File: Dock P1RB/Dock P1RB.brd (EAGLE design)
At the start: 41 x 46 mm, 16 parts, among them U1 MCP73831T-2ACI/OT

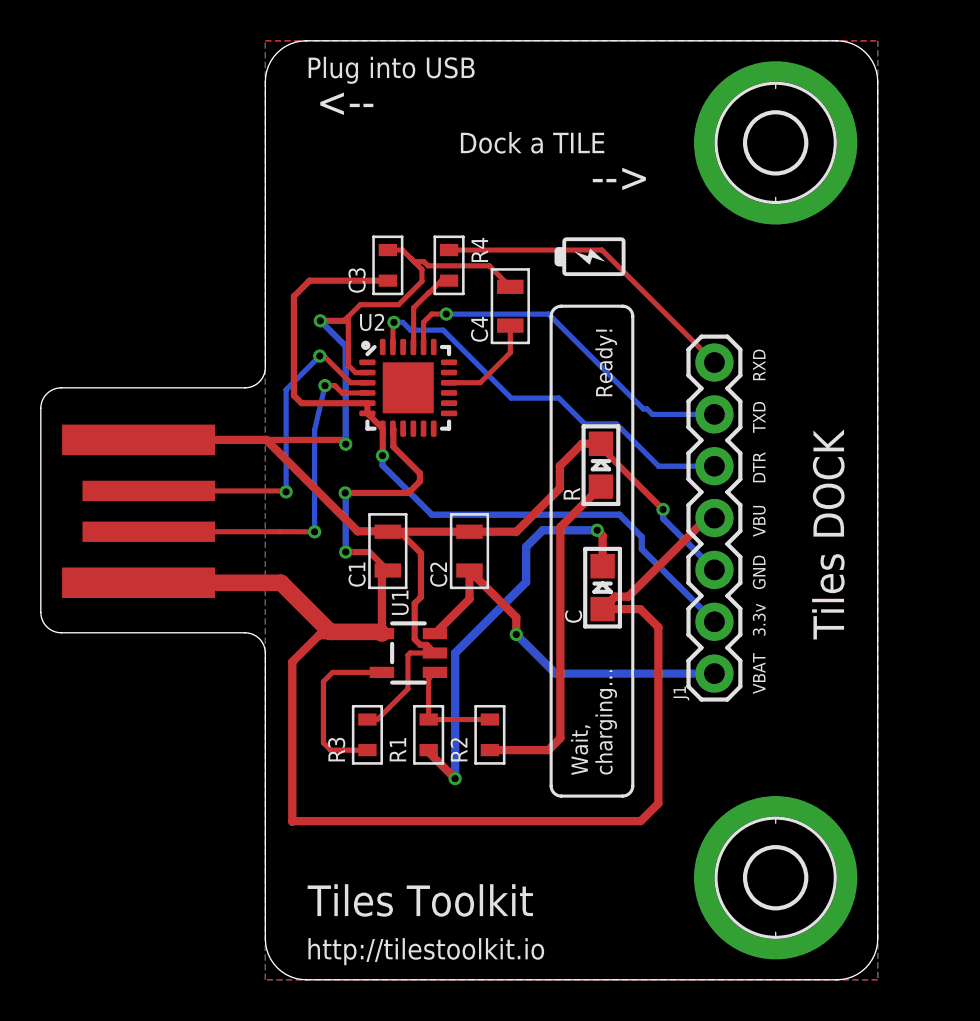
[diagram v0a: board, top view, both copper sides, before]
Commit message: dock ready for prod
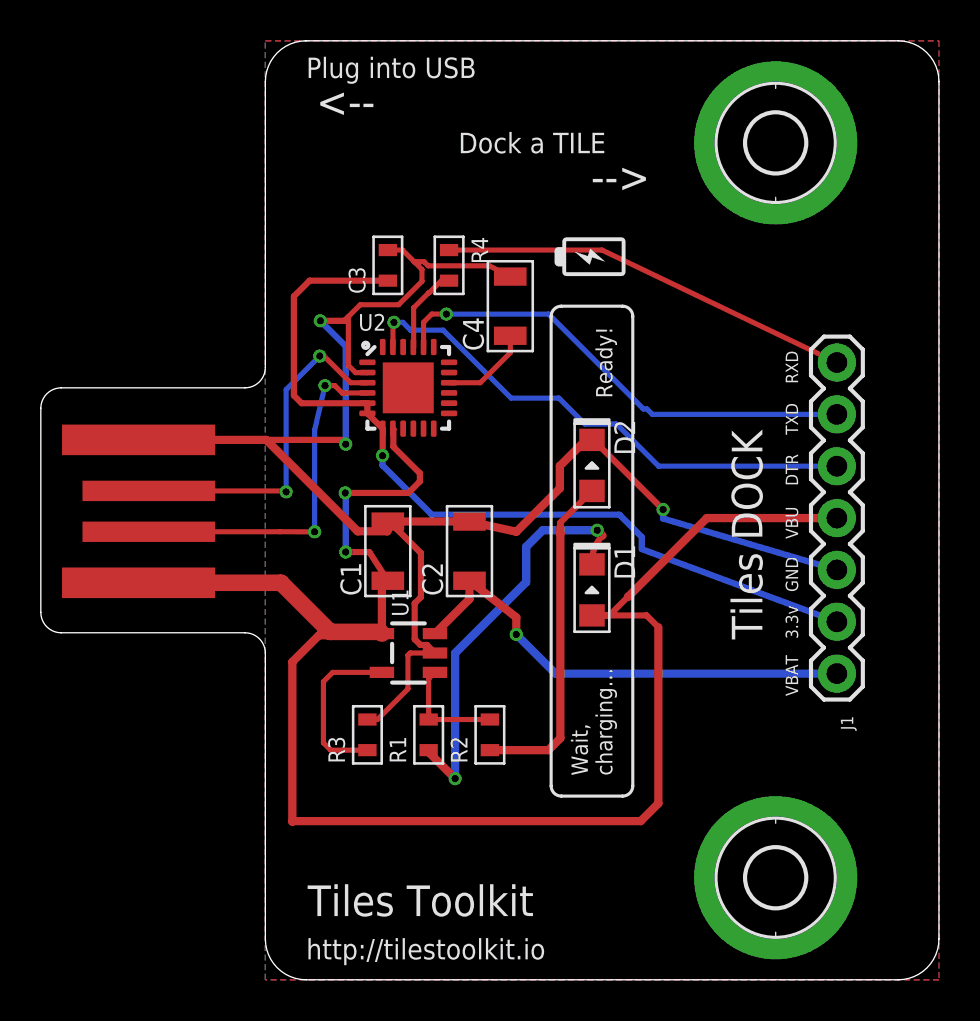
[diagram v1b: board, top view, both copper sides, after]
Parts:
- removed C: RED, microbuilder:CHIPLED_0805
- removed R: GREEN, microbuilder:CHIPLED_0805
- added D1: MF-LED-0805-RED, MF_LEDs:LED0805
- added D2: MF-LED-0805-GREEN, MF_LEDs:LED0805
- C1, C2, C4: device MF_Passives:C0805 -> MF_Passives:C1206
- moved J1 6.00 mm to (28.0, -31.0)
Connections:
- net GND: now also D2.CATHODE; no longer R.C
- net N$1: now also D1.CATHODE; no longer C.C
- net N$6: now also D2.ANODE; no longer R.A
- net VBUS: now also D1.ANODE; no longer C.A
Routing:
- net VBUS: track 76.2 -> 83.6 mm
- net TXD: track 17.7 -> 23.7 mm
- net DTR: track 19.8 -> 25.8 mm
- net VBAT: track 18.4 -> 23.5 mm
- net 3.3V: track 36.7 -> 41.8 mm
- net RXD: track 15.3 -> 20.3 mm
- net GND: track 76.6 -> 81.0 mm
- net N$3: track 4.94 -> 4.44 mm
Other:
- board size 41 x 46 mm -> 44 x 46 mm
- board text added: "Tiles IoT Dock"
